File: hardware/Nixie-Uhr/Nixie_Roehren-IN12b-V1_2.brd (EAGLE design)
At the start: 158.5 x 48 mm, 30 parts

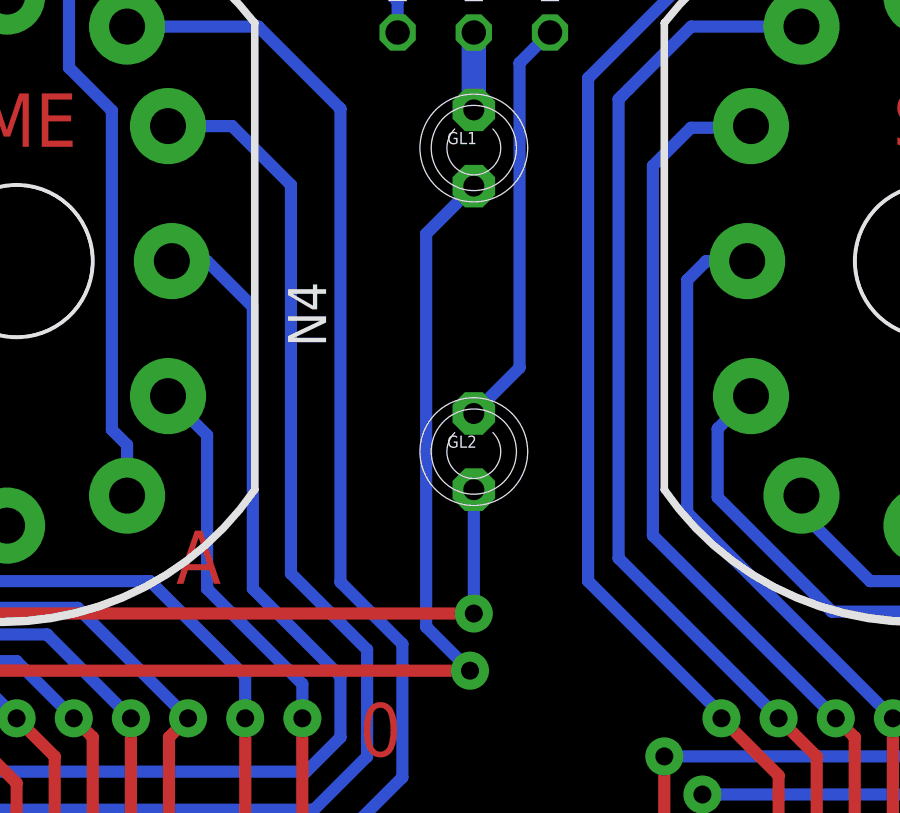
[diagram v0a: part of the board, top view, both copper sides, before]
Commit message: Hardware description updated.
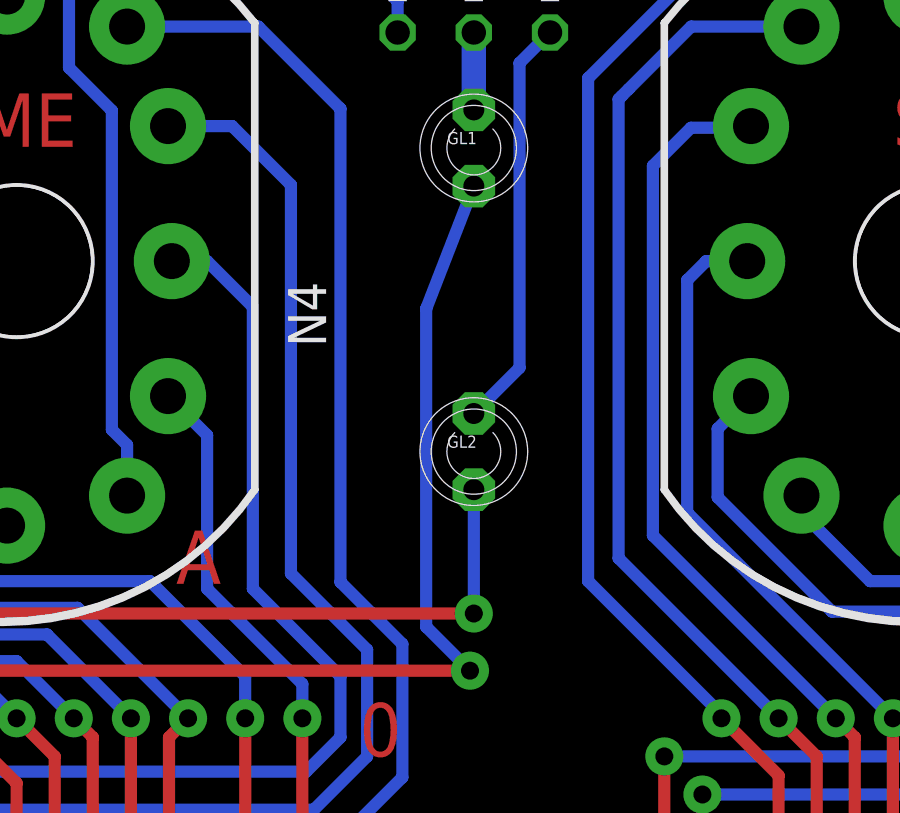
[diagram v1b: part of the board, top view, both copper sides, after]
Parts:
- R10, R7, R8, R9: value 56k -> 220k
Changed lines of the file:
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@@
 <?xml version="1.0" encoding="utf-8"?>
 <!DOCTYPE eagle SYSTEM "eagle.dtd">
-<eagle version="7.6.0">
+<eagle version="7.7.0">
 <drawing>
 <settings>
@@
 <layer number="17" name="Pads" color="2" fill="1" visible="yes" active="yes"/>
 <layer number="18" name="Vias" color="2" fill="1" visible="yes" active="yes"/>
-<layer number="19" name="Unrouted" color="6" fill="1" visible="yes" active="yes"/>
+<layer number="19" name="Unrouted" color="6" fill="1" visible="no" active="yes"/>
 <layer number="20" name="Dimension" color="15" fill="1" visible="yes" active="yes"/>
 <layer number="21" name="tPlace" color="7" fill="1" visible="yes" active="yes"/>
@@
 <dimension x1="68.58" y1="28.48" x2="0" y2="57.35" x3="34.29" y3="57.6" textsize="1.778" layer="47" dtype="horizontal"/>
 <dimension x1="90.17" y1="28.48" x2="0" y2="60.7" x3="45.085" y3="60.7" textsize="1.778" layer="47" dtype="horizontal"/>
-<dimension x1="105.41" y1="32.25" x2="0" y2="59.95" x3="52.705" y3="63.7" textsize="1.778" layer="47" dtype="horizontal"/>
+<dimension x1="105.41" y1="29.75" x2="0" y2="59.95" x3="52.705" y3="63.7" textsize="1.778" layer="47" dtype="horizontal"/>
 <dimension x1="120.65" y1="28.48" x2="0" y2="66.6" x3="60.325" y3="66.75" textsize="1.778" layer="47" dtype="horizontal"/>
 <dimension x1="142.24" y1="28.48" x2="0" y2="70.05" x3="71.12" y3="69.9" textsize="1.778" layer="47" dtype="horizontal"/>
@@
 <text x="148.59" y="1.905" size="1.778" layer="16" font="vector" ratio="12" rot="MR0">1</text>
 <dimension x1="0" y1="0" x2="20.32" y2="5.62" x3="-1" y3="2.81" textsize="1.778" layer="47" dtype="vertical"/>
-<dimension x1="0" y1="0" x2="53.34" y2="32.25" x3="-15.1" y3="16.125" textsize="1.778" textratio="12" layer="47" dtype="vertical"/>
 <dimension x1="0" y1="0" x2="53.34" y2="22.13" x3="-8.8" y3="11.065" textsize="1.778" textratio="12" layer="47" dtype="vertical"/>
+<dimension x1="0" y1="0" x2="53.34" y2="32.25" x3="-15" y3="16.125" textsize="1.778" layer="47" dtype="vertical"/>
 </plain>
 <attributes>
@@
 <element name="R5" library="rcl" package="0207/10" value="27k" x="50.8" y="41.18" rot="R90"/>
 <element name="R6" library="rcl" package="0207/10" value="27k" x="26.67" y="41.18" rot="R90"/>
-<element name="R7" library="rcl" package="0207/10" value="56k" x="105.41" y="41.18" rot="R90"/>
-<element name="R8" library="rcl" package="0207/10" value="56k" x="107.95" y="41.18" rot="R90"/>
-<element name="R9" library="rcl" package="0207/10" value="56k" x="53.34" y="41.18" rot="R90"/>
-<element name="R10" library="rcl" package="0207/10" value="56k" x="55.88" y="41.18" rot="R90"/>
+<element name="R7" library="rcl" package="0207/10" value="220k" x="105.41" y="41.18" rot="R90"/>
+<element name="R8" library="rcl" package="0207/10" value="220k" x="107.95" y="41.18" rot="R90"/>
+<element name="R9" library="rcl" package="0207/10" value="220k" x="53.34" y="41.18" rot="R90"/>
+<element name="R10" library="rcl" package="0207/10" value="220k" x="55.88" y="41.18" rot="R90"/>
 <element name="N1" library="russian-nixies" package="IN-12" value="IN-12B" x="38.1" y="28.48"/>
 <element name="N2" library="russian-nixies" package="IN-12" value="IN-12B" x="16.51" y="28.48"/>
@@
 <wire x1="52.07" y1="14.8275" x2="105.283" y2="14.8275" width="0.4064" layer="1"/>
 <via x="105.283" y="14.8275" extent="1-16" drill="0.6" diameter="1.27"/>
-<wire x1="103.8225" y1="29.3925" x2="103.8225" y2="16.288" width="0.4064" layer="16"/>
+<wire x1="105.41" y1="30.98" x2="103.8225" y2="26.8925" width="0.4064" layer="16"/>
+<wire x1="103.8225" y1="26.8925" x2="103.8225" y2="16.288" width="0.4064" layer="16"/>
 <wire x1="105.283" y1="14.8275" x2="103.8225" y2="16.288" width="0.4064" layer="16"/>
-<wire x1="103.8225" y1="29.3925" x2="105.41" y2="30.98" width="0.4064" layer="16"/>
 </signal>
 <signal name="DP1">
